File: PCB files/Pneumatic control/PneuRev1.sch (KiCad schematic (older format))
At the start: 72 parts, among them J1 SIG_IN, J2 BATT_IN, J3 PNEU, U1 OPA551, U10 OPA551, U11 OPA551, U12 OPA551, U13 OPA551, U2 OPA551, U3 OPA551, U4 OPA551, U5 OPA551, U6 OPA551, U7 OPA551, U8 OPA551, U9 OPA551

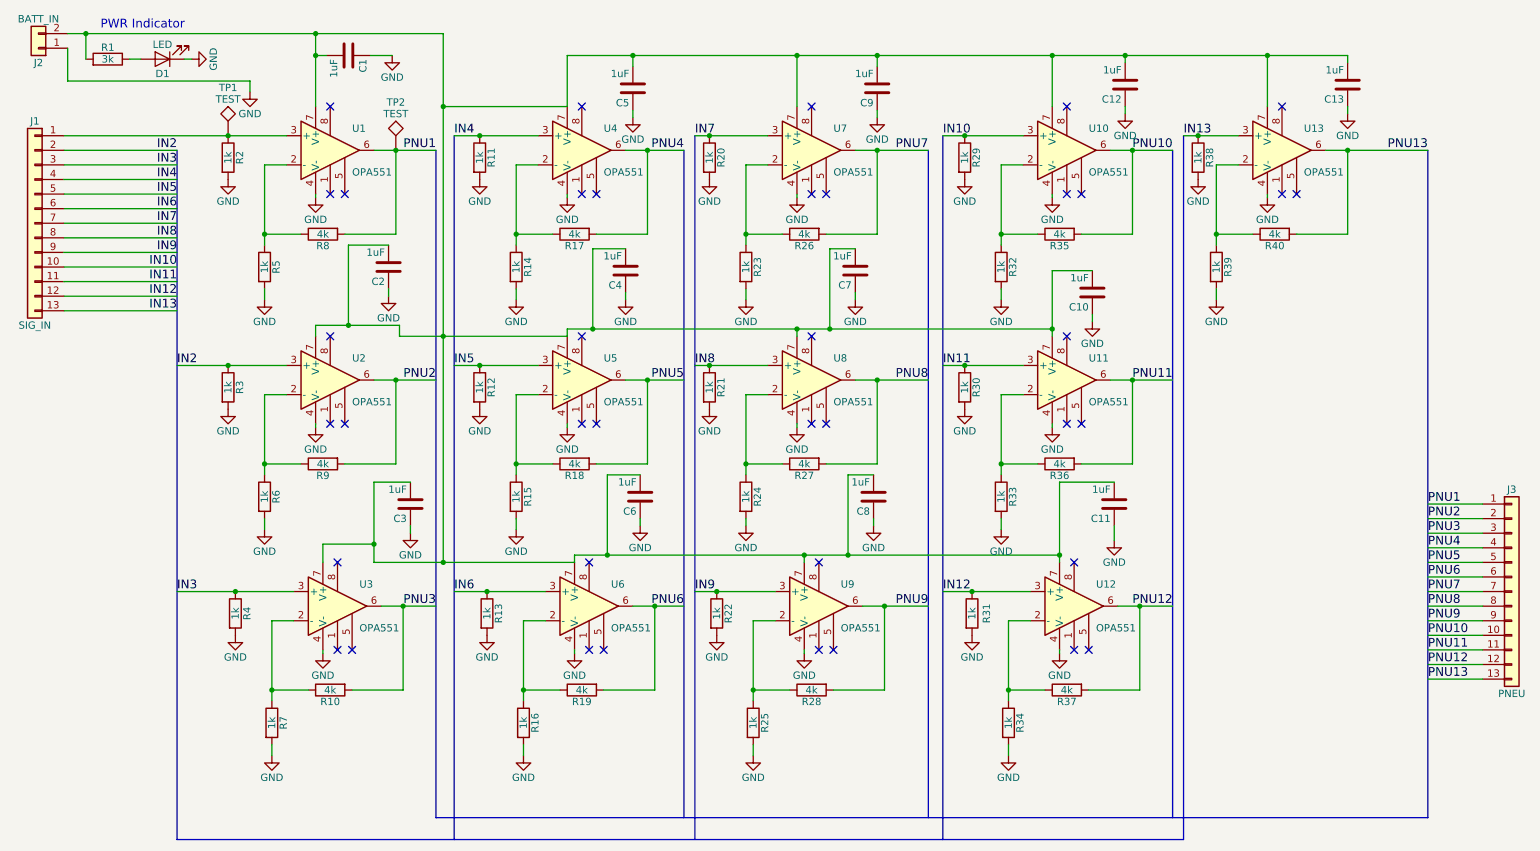
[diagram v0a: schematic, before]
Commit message: 8/2/2019 Formatted w/Hierarchies
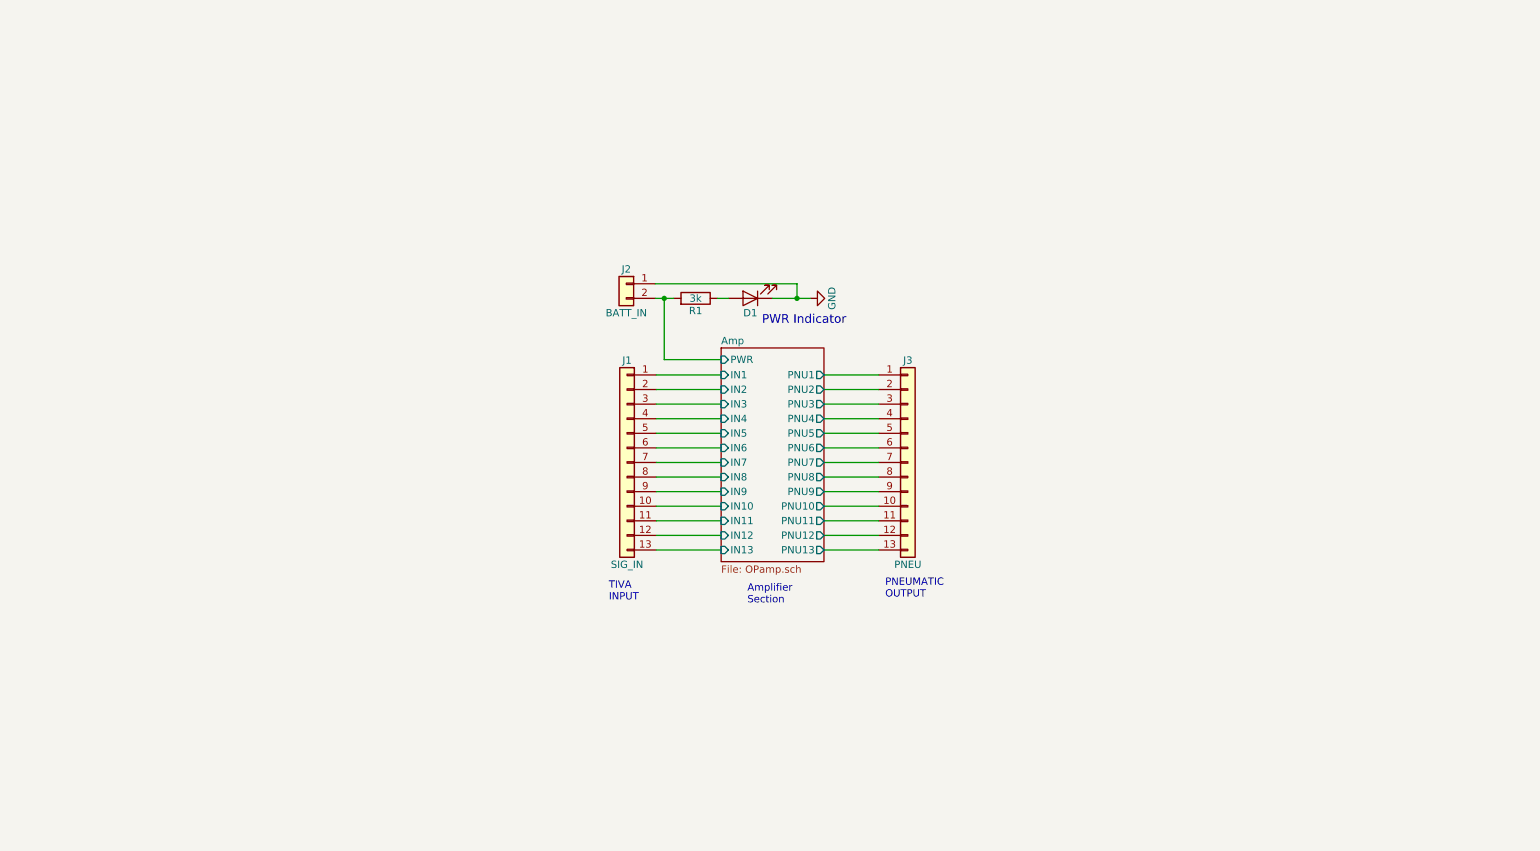
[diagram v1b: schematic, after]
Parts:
- removed C1, C10, C11, C12, C13, C2, C3, C4, C5, C6, C7, C8, C9: 1uF, Capacitors_THT:C_Disc_D3.4mm_W2.1mm_P2.50mm, symbol Device:C
- removed R10, R8, R9: 4k, Resistors_THT:R_Axial_DIN0309_L9.0mm_D3.2mm_P12.70mm_Horizontal, symbol Device:R
- removed R11, R12, R13, R14, R15, R16, R2, R20, R21, R22, R23, R24, R25, R29, R3, R30, R31, R32, R33, R34, R38, R39, R4, R5, R6, R7: 1k, Resistors_THT:R_Axial_DIN0204_L3.6mm_D1.6mm_P5.08mm_Horizontal, symbol Device:R
- removed R17, R18, R19, R26, R27, R28, R35, R36, R37: 4k, Resistors_THT:R_Axial_DIN0411_L9.9mm_D3.6mm_P12.70mm_Horizontal, symbol Device:R
- removed R40: 4k, Resistors_THT:R_Axial_DIN0204_L3.6mm_D1.6mm_P5.08mm_Horizontal, symbol Device:R
- removed TP1, TP2: TEST, Measurement_Points:Measurement_Point_Round-SMD-Pad_Big, symbol PneuRev1-rescue:TEST
- removed U1, U10, U11, U12, U13, U2, U3, U4, U5, U6, U7, U8, U9: OPA551, Housings_DIP:DIP-8_W7.62mm, symbol PneuRev1-rescue:OPA551
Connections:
- net Amp/IN1: now reaches J1.1 (Pin_1)
- net Amp/PWR: now reaches J2.2 (Pin_2), R1.2
- net IN10 renamed Amp/IN10
- net IN11 renamed Amp/IN11
- net IN12 renamed Amp/IN12
- net IN13 renamed Amp/IN13
- net IN2 renamed Amp/IN2
- net IN3 renamed Amp/IN3
- net IN4 renamed Amp/IN4
- net IN5 renamed Amp/IN5
- net IN6 renamed Amp/IN6
- net IN7 renamed Amp/IN7
- net IN8 renamed Amp/IN8
- net IN9 renamed Amp/IN9
- net PNU1 renamed Amp/PNU1
- net PNU10 renamed Amp/PNU10
- net PNU11 renamed Amp/PNU11
- net PNU12 renamed Amp/PNU12
- net PNU13 renamed Amp/PNU13
- net PNU2 renamed Amp/PNU2
- net PNU3 renamed Amp/PNU3
- net PNU4 renamed Amp/PNU4
- net PNU5 renamed Amp/PNU5
- net PNU6 renamed Amp/PNU6
- net PNU7 renamed Amp/PNU7
- net PNU8 renamed Amp/PNU8
- net PNU9 renamed Amp/PNU9
- no-connect marks 39 -> 0
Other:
- note added: "Amplifier\nSection"
- note added: "PNEUMATIC\nOUTPUT"
- note added: "TIVA\nINPUT"
- moved on the sheet: D1, J1, J2, J3, R1
